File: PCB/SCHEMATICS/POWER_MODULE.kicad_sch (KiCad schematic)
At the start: 36 parts, among them Q1 PMOS, U1 C7433, U2 AMS1117-3.3

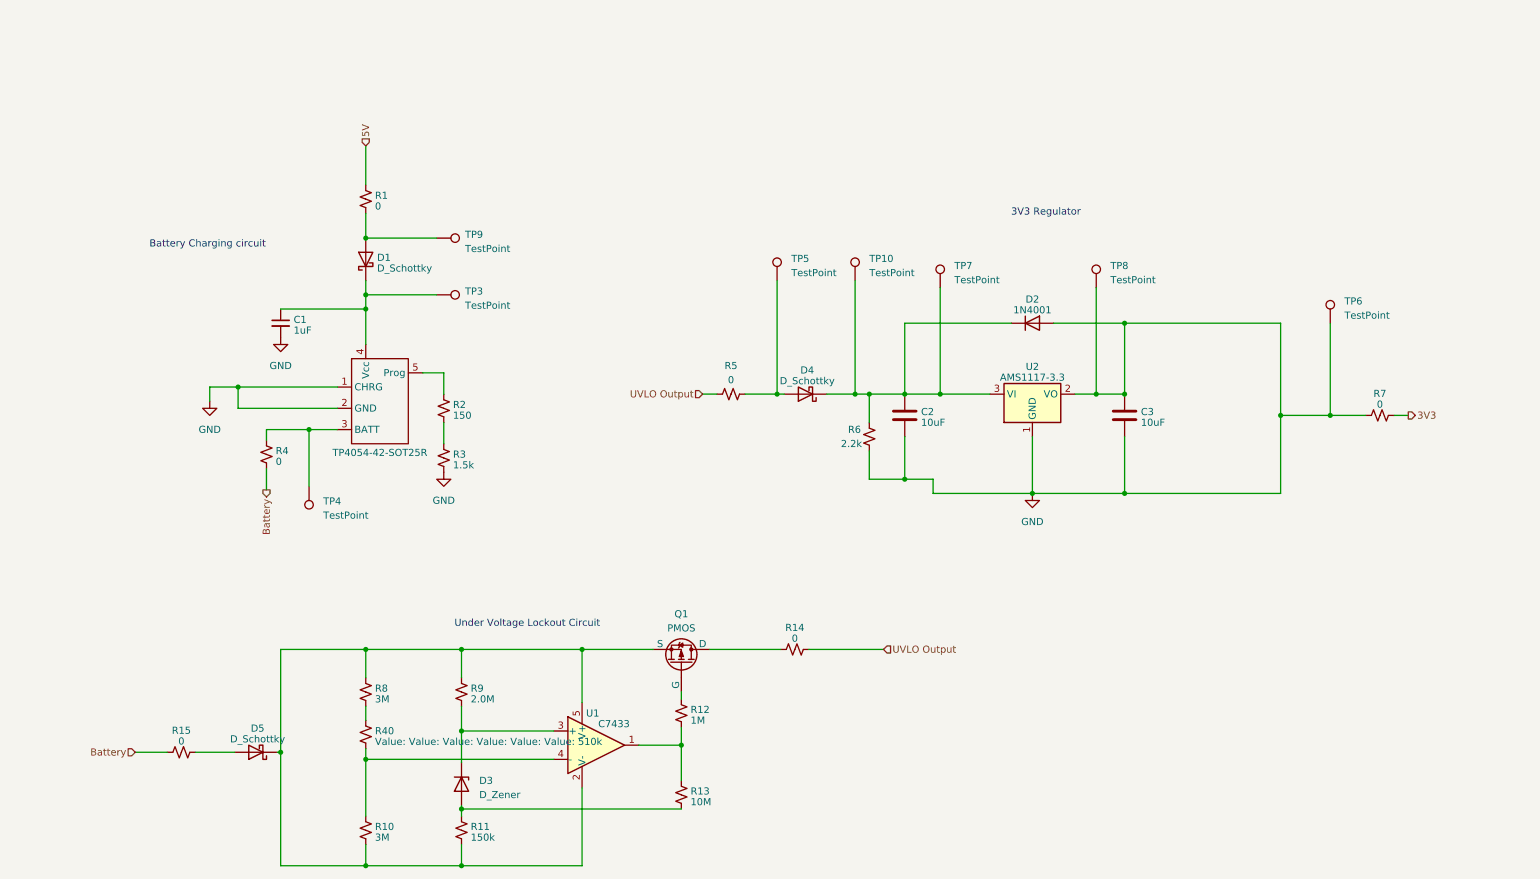
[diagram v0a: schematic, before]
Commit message: Updating schematics
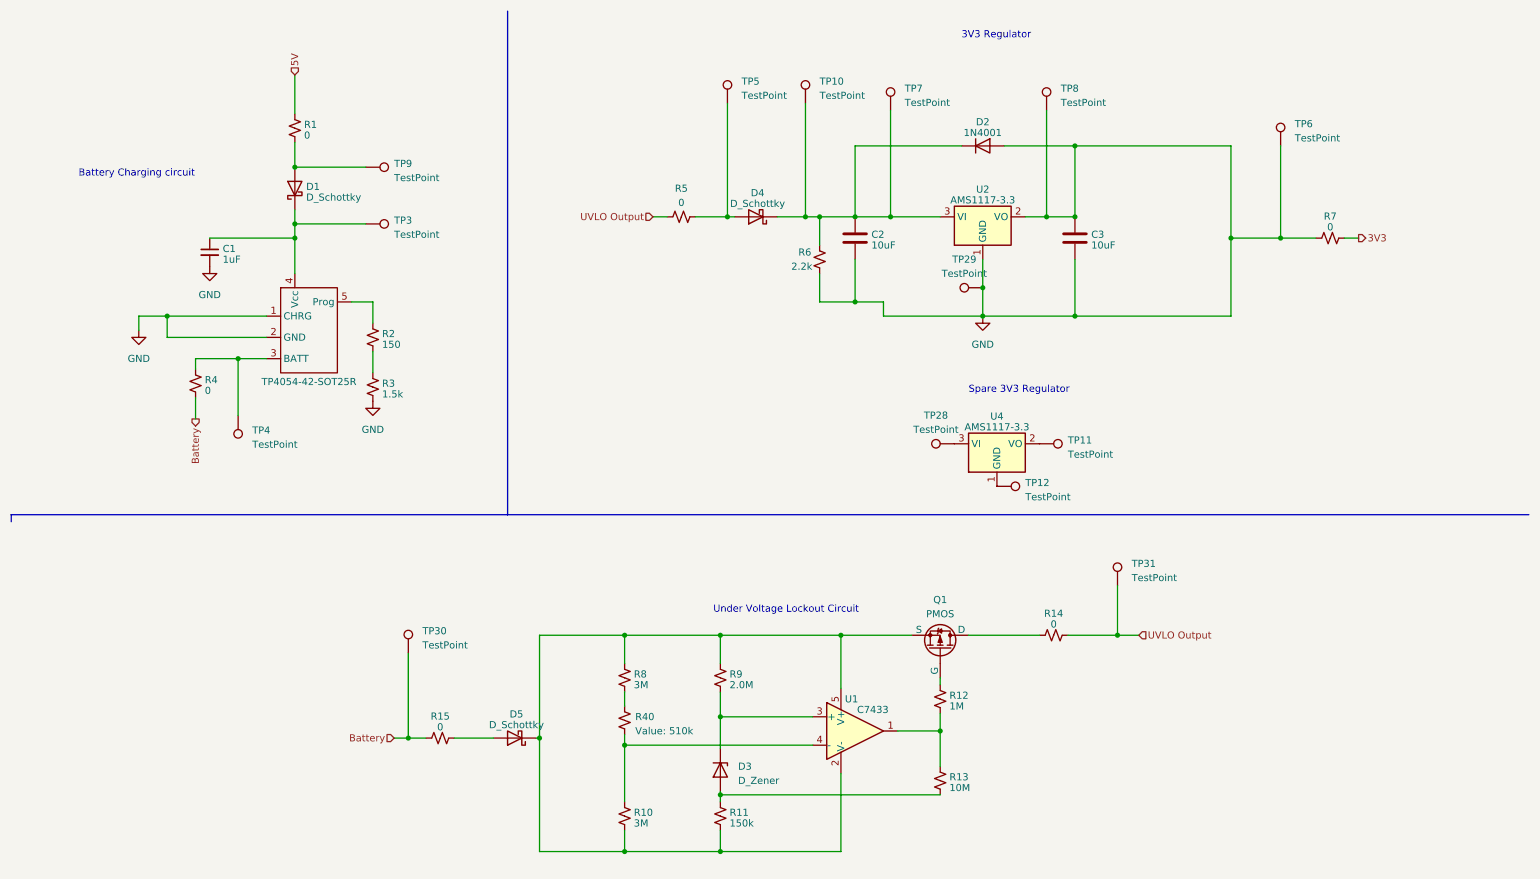
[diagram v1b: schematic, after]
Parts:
- added TP11, TP12, TP28, TP29, TP30, TP31: TestPoint, symbol Connector:TestPoint
- added U4: AMS1117-3.3, Package_TO_SOT_SMD:SOT-223-3_TabPin2, symbol Regulator_Linear:AMS1117-3.3
- R40: value Value: Value: Value: Value: Value: 510k -> 510k
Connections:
- net Battery: now also TP30.1
- net GND: now also TP29.1
- net UVLO Output: now also TP31.1
- new net: TP28.1, U4.3 (VI)
- new net: TP11.1, U4.2 (VO)
- new net: TP12.1, U4.1 (GND)
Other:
- note added: "Spare 3V3 Regulator"
- moved on the sheet: C1, C2, C3, D1, D2, D3, D4, D5, Q1, R1, R10, R11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
